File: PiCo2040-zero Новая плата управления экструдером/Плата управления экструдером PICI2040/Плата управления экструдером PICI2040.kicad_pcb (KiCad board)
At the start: 2 copper layers, 100.2 x 42 mm, 32 parts, among them J10 Conn_01x08_Pin, J5 Conn_01x08_Pin, J6 Conn_01x08_Pin, J7 Conn_01x08_Pin, J8 Conn_01x08_Pin, J9 Conn_02x03_Odd_Even, Q1 IRLB8721, Q2 IRLB8721, Q3 IRLB8721, U1 rp2040-zero

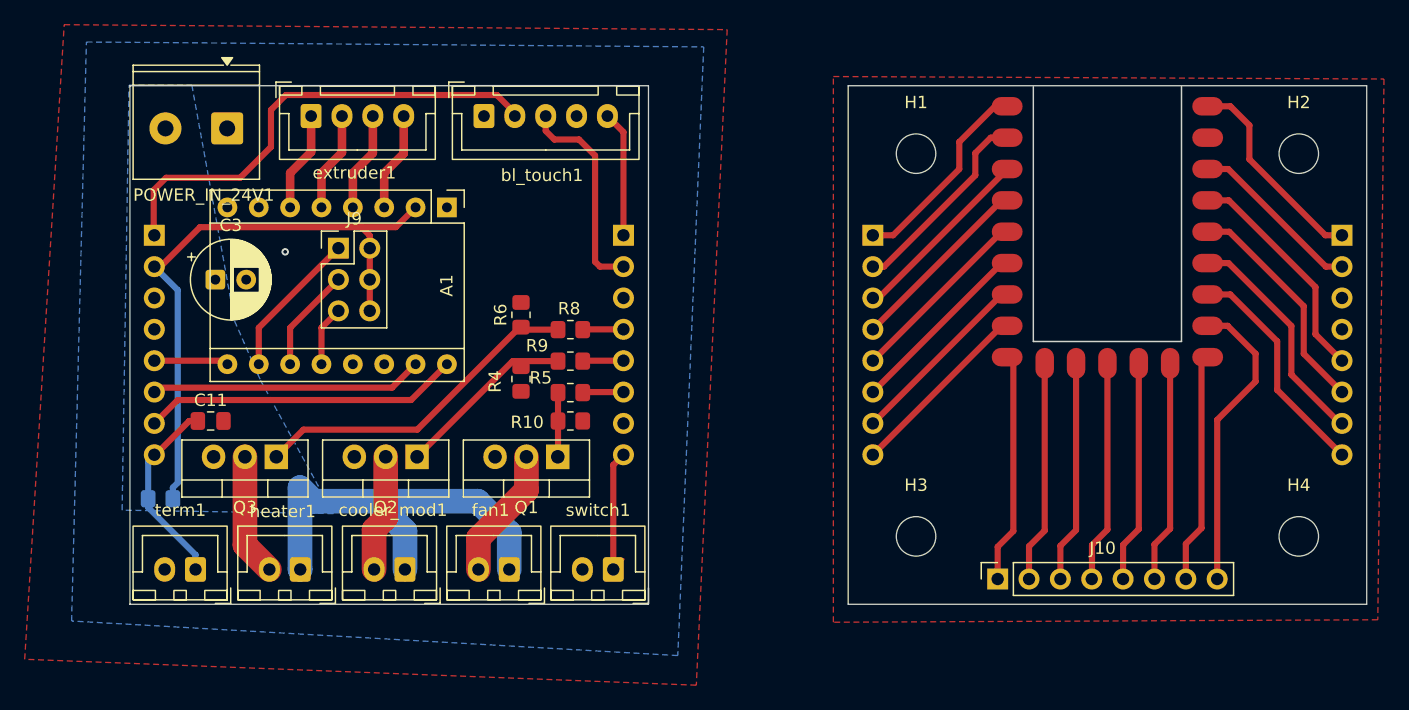
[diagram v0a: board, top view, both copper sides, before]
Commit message: Мелкие правки платы
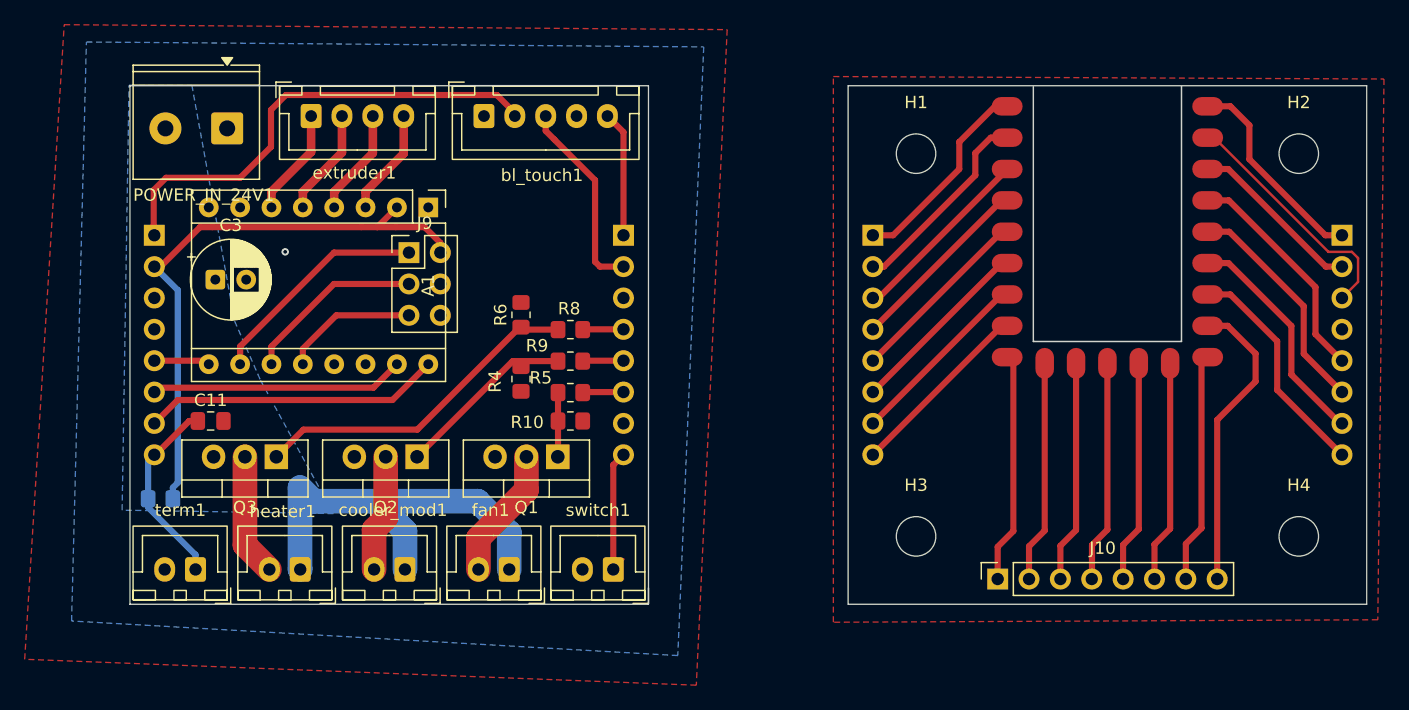
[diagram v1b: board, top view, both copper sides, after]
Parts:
- moved J9 5.73 mm to (124.4, 91.1)
- moved A1 1.51 mm to (126.0, 87.4)
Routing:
- net GND: track 0.04 -> 20.5 mm
- net Net-(A1-MS3): track 5.05 -> 11.3 mm
- net Net-(A1-MS1): track 12.2 -> 18.3 mm
- net Net-(A1-MS2): track 8.64 -> 14.7 mm
- net +3.3V: track 64.0 -> 61.9 mm
- net /DIR_PB: track 25.7 -> 24.2 mm
- net /STEP_PB: track 22.1 -> 20.6 mm
- net /ENABLE_PB: track 6.19 -> 4.69 mm
- net /BL_contr_signal_PB: track 17.1 -> 15.9 mm
- net Net-(A1-2A): track 7.64 -> 8.26 mm
- net Net-(A1-1B): track 7.60 -> 8.23 mm
- net Net-(A1-2B): track 7.65 -> 8.28 mm
- net Net-(A1-1A): track 7.62 -> 8.25 mm

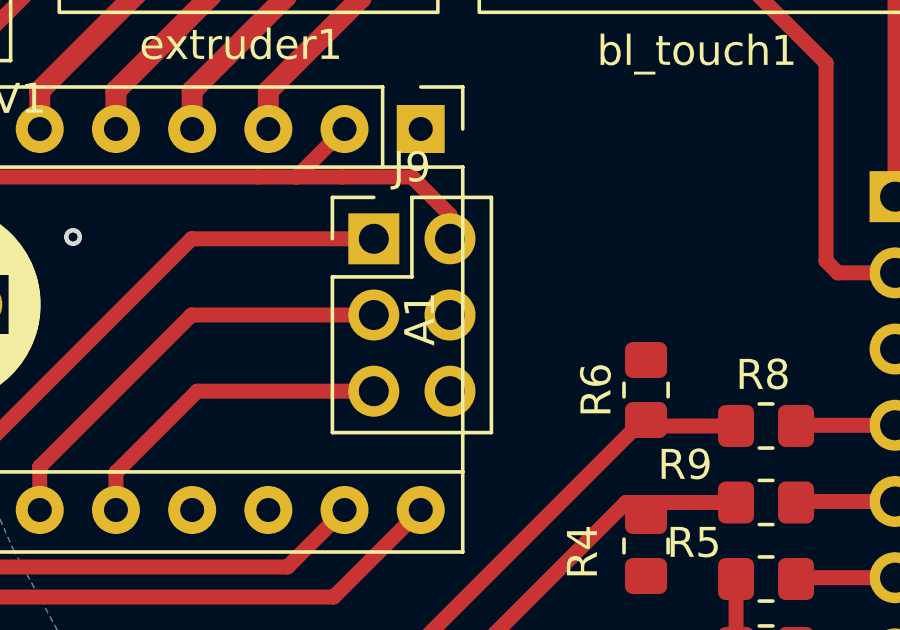
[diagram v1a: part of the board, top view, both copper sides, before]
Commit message: Механика гравера
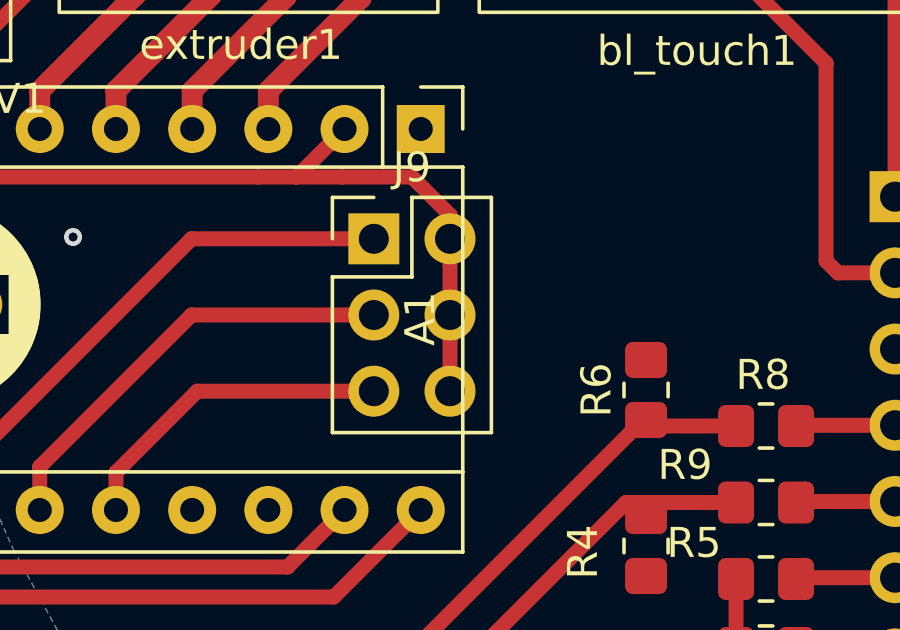
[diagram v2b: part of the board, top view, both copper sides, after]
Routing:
- net +3.3V: track 61.9 -> 66.9 mm
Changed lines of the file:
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@@
+	)
+	(segment
+		(start 126.965 91.06)
+		(end 126.965 93.6)
+		(width 0.5)
+		(layer "F.Cu")
+		(net "+3.3V")
 	)
 	(segment
@@
 		(width 0.5)
 		(layer "F.Cu")
+		(net "+3.3V")
+	)
+	(segment
+		(start 126.965 93.6)
+		(end 126.965 96.14)
+		(width 0.5)
+		(layer "F.Cu")
